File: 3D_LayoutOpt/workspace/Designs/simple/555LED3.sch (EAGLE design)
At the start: 10 parts, among them IC1 555, IC2 555, IC3 555, IC4 555

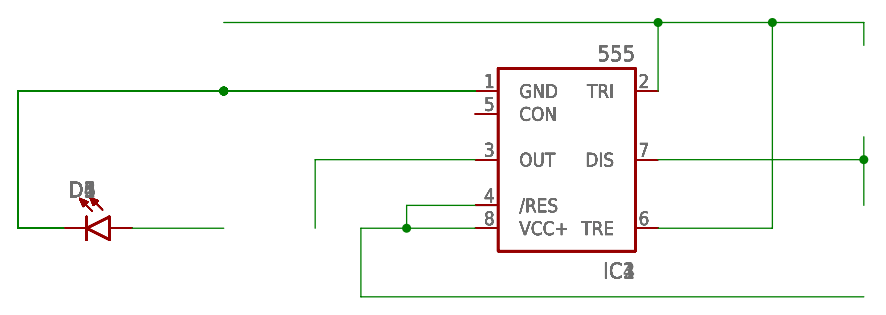
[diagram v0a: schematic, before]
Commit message: Code works!
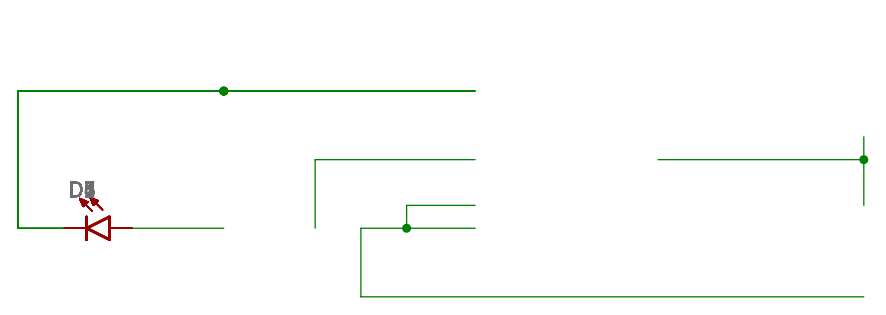
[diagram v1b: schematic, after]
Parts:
- removed IC1, IC2, IC3, IC4: 555, SparkFun-IC-Special-Function:555D
- added D7: (no value), SparkFun-LED:LED1206
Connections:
- removed net N$7: D1.C, D4.A, IC2.DIS
- removed net N$8: D3.A, D6.C, IC1.GND, IC2.OUT, IC3.DIS
- net N$1: now also D1.A; no longer IC1.OUT
- net N$2: now also D3.C; no longer IC2.GND
- net N$3: now also D2.A, D5.C; no longer IC1./RES, IC4.VCC+
- net N$4: now also D6.A, D7.A; no longer D5.A, IC3.GND
- net N$5: now also D2.C, D3.A; no longer D5.A, IC1.TRI, IC3.TRE
- net N$6: now also D4.C, D5.A, D7.A; no longer D4.A, IC2.GND
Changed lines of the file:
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@@
 </classes>
 <parts>
-<part name="IC1" library="SparkFun-IC-Special-Function" deviceset="555" device="D" value="555"/>
-<part name="IC2" library="SparkFun-IC-Special-Function" deviceset="555" device="D" value="555"/>
-<part name="IC3" library="SparkFun-IC-Special-Function" deviceset="555" device="D" value="555"/>
-<part name="IC4" library="SparkFun-IC-Special-Function" deviceset="555" device="D" value="555"/>
 <part name="D1" library="SparkFun-LED" deviceset="LED" device="1206"/>
 <part name="D2" library="SparkFun-LED" deviceset="LED" device="1206"/>
@@
 <part name="D5" library="SparkFun-LED" deviceset="LED" device="1206"/>
 <part name="D6" library="SparkFun-LED" deviceset="LED" device="1206"/>
+<part name="D7" library="SparkFun-LED" deviceset="LED" device="1206"/>
 </parts>
 <sheets>
@@
 </plain>
 <instances>
-<instance part="IC1" gate="G$1" x="50.8" y="58.42" rot="R180"/>
-<instance part="IC2" gate="G$1" x="50.8" y="58.42" rot="R180"/>
-<instance part="IC3" gate="G$1" x="50.8" y="58.42" rot="R180"/>
-<instance part="IC4" gate="G$1" x="50.8" y="58.42" rot="R180"/>
 <instance part="D1" gate="G$1" x="0" y="50.8" rot="R270"/>
 <instance part="D2" gate="G$1" x="0" y="50.8" rot="R270"/>
@@
 <instance part="D5" gate="G$1" x="0" y="50.8" rot="R270"/>
 <instance part="D6" gate="G$1" x="0" y="50.8" rot="R270"/>
+<instance part="D7" gate="G$1" x="0" y="50.8" rot="R270"/>
 </instances>
 <busses>
@@
 <net name="N$1" class="0">
 <segment>
-<pinref part="IC1" gate="G$1" pin="OUT"/>
+<pinref part="D1" gate="G$1" pin="A"/>
 <pinref part="D3" gate="G$1" pin="A"/>
 <wire x1="40.64" y1="58.42" x2="22.86" y2="58.42" width="0.1524" layer="91"/>
@@
 <net name="N$2" class="0">
 <segment>
-<pinref part="IC2" gate="G$1" pin="GND"/>
+<pinref part="D3" gate="G$1" pin="C"/>
 <pinref part="D1" gate="G$1" pin="A"/>
 <pinref part="D2" gate="G$1" pin="C"/>
@@
 <net name="N$3" class="0">
 <segment>
-<pinref part="IC1" gate="G$1" pin="/RES"/>
+<pinref part="D4" gate="G$1" pin="A"/>
 <wire x1="40.64" y1="53.34" x2="33.02" y2="53.34" width="0.1524" layer="91"/>
 <wire x1="33.02" y1="53.34" x2="33.02" y2="50.8" width="0.1524" layer="91"/>
-<pinref part="IC4" gate="G$1" pin="VCC+"/>
+<pinref part="D5" gate="G$1" pin="C"/>
 <wire x1="33.02" y1="50.8" x2="40.64" y2="50.8" width="0.1524" layer="91"/>
-<pinref part="D4" gate="G$1" pin="A"/>
+<pinref part="D2" gate="G$1" pin="A"/>
 <wire x1="83.82" y1="43.18" x2="27.94" y2="43.18" width="0.1524" layer="91"/>
 <wire x1="27.94" y1="43.18" x2="27.94" y2="50.8" width="0.1524" layer="91"/>
@@
 </segment>
 </net>
-<net name="N$5" class="0">
-<segment>
-<pinref part="IC1" gate="G$1" pin="TRI"/>
-<wire x1="60.96" y1="73.66" x2="60.96" y2="66.04" width="0.1524" layer="91"/>
-<pinref part="D5" gate="G$1" pin="A"/>
-<wire x1="60.96" y1="73.66" x2="73.66" y2="73.66" width="0.1524" layer="91"/>
-<wire x1="73.66" y1="73.66" x2="83.82" y2="73.66" width="0.1524" layer="91"/>
-<wire x1="83.82" y1="73.66" x2="83.82" y2="71.12" width="0.1524" layer="91"/>
-<pinref part="IC3" gate="G$1" pin="TRE"/>
-<wire x1="60.96" y1="50.8" x2="73.66" y2="50.8" width="0.1524" layer="91"/>
-<wire x1="73.66" y1="50.8" x2="73.66" y2="73.66" width="0.1524" layer="91"/>
-<junction x="73.66" y="73.66"/>
-<pinref part="D6" gate="G$1" pin="C"/>
-<wire x1="12.7" y1="73.66" x2="60.96" y2="73.66" width="0.1524" layer="91"/>
-<junction x="60.96" y="73.66"/>
-</segment>
-</net>
-<net name="N$7" class="0">
+<net name="N$4" class="0">
 <segment>
 <pinref part="D1" gate="G$1" pin="C"/>
-<pinref part="D4" gate="G$1" pin="A"/>
+<pinref part="D6" gate="G$1" pin="A"/>
 <wire x1="83.82" y1="60.96" x2="83.82" y2="58.42" width="0.1524" layer="91"/>
-<pinref part="IC2" gate="G$1" pin="DIS"/>
+<pinref part="D7" gate="G$1" pin="A"/>
 <wire x1="83.82" y1="58.42" x2="83.82" y2="53.34" width="0.1524" layer="91"/>
 <wire x1="60.96" y1="58.42" x2="83.82" y2="58.42" width="0.1524" layer="91"/>
@@
 </segment>
 </net>
-<net name="N$4" class="0">
+<net name="N$5" class="0">
 <segment>
-<pinref part="D1" gate="G$1" pin="C"/>
+<pinref part="D2" gate="G$1" pin="C"/>
 <wire x1="-5.08" y1="50.8" x2="-10.16" y2="50.8" width="0.1524" layer="91"/>
 <wire x1="-10.16" y1="50.8" x2="-10.16" y2="66.04" width="0.1524" layer="91"/>
-<pinref part="D5" gate="G$1" pin="A"/>
+<pinref part="D3" gate="G$1" pin="A"/>
 <wire x1="-10.16" y1="66.04" x2="12.7" y2="66.04" width="0.1524" layer="91"/>
-<pinref part="IC3" gate="G$1" pin="GND"/>
+<pinref part="D6" gate="G$1" pin="C"/>
 <wire x1="12.7" y1="66.04" x2="40.64" y2="66.04" width="0.1524" layer="91"/>
 <junction x="12.7" y="66.04"/>
@@
 <wire x1="-5.08" y1="50.8" x2="-10.16" y2="50.8" width="0.1524" layer="91"/>
 <wire x1="-10.16" y1="50.8" x2="-10.16" y2="66.04" width="0.1524" layer="91"/>
-<pinref part="D4" gate="G$1" pin="A"/>
+<pinref part="D5" gate="G$1" pin="A"/>
 <wire x1="-10.16" y1="66.04" x2="12.7" y2="66.04" width="0.1524" layer="91"/>
-<pinref part="IC2" gate="G$1" pin="GND"/>
+<pinref part="D7" gate="G$1" pin="A"/>
+<pinref part="D4" gate="G$1" pin="C"/>
 <wire x1="12.7" y1="66.04" x2="40.64" y2="66.04" width="0.1524" layer="91"/>
 <junction x="12.7" y="66.04"/>
-</segment>
-</net>
-<net name="N$8" class="0">
-<segment>
-<pinref part="D6" gate="G$1" pin="C"/>
-<wire x1="-5.08" y1="50.8" x2="-10.16" y2="50.8" width="0.1524" layer="91"/>
-<wire x1="-10.16" y1="50.8" x2="-10.16" y2="66.04" width="0.1524" layer="91"/>
-<pinref part="D3" gate="G$1" pin="A"/>
-<wire x1="-10.16" y1="66.04" x2="12.7" y2="66.04" width="0.1524" layer="91"/>
-<pinref part="IC1" gate="G$1" pin="GND"/>
-<pinref part="IC2" gate="G$1" pin="OUT"/>
-<pinref part="IC3" gate="G$1" pin="DIS"/>
-<wire x1="12.7" y1="66.04" x2="40.64" y2="66.04" width="0.1524" layer="91"/>
-<junction x="12.7" y="66.04"/>
